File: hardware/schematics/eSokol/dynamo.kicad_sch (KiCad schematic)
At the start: 4 parts, among them U4 AMS1117-5.0

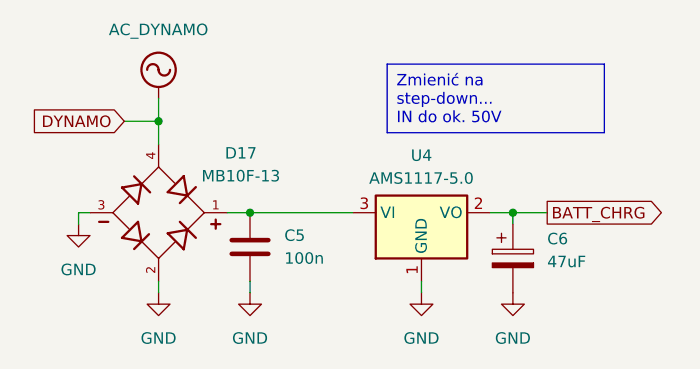
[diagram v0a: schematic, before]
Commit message: WIP: update some schematics to reflect the newest design changes
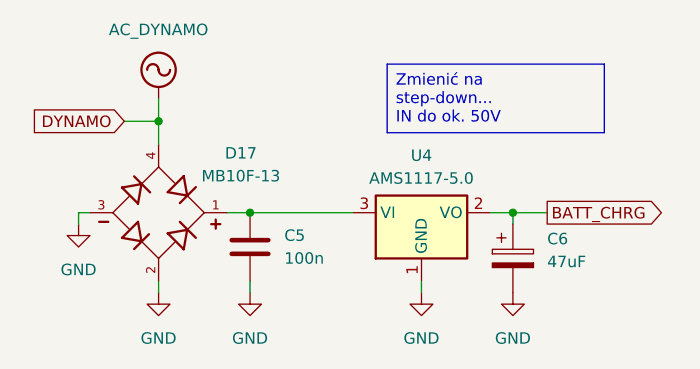
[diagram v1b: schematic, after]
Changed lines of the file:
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@@
 (kicad_sch
-	(version 20231120)
+	(version 20250114)
 	(generator "eeschema")
-	(generator_version "8.0")
+	(generator_version "9.0")
 	(paper "A4")
+	(text_box "Zmienić na step-down...\nIN do ok. 50V"
+		(exclude_from_sim no)
+		(at 115.57 69.85 0)
+		(size 24.13 7.62)
+		(margins 0.9525 0.9525 0.9525 0.9525)
+		(stroke
+			(width 0)
+			(type default)
+		)
+		(fill
+			(type none)
+		)
+		(effects
+			(font
+				(size 1.27 1.27)
+			)
+			(justify left top)
+		)
+	)
 	(junction
 		(at 129.54 86.36)
@@
 		)
 	)
-	(text_box "Zmienić na step-down...\nIN do ok. 50V"
-		(exclude_from_sim no)
-		(at 115.57 69.85 0)
-		(size 24.13 7.62)
-		(stroke
-			(width 0)
-			(type default)
-		)
-		(fill
-			(type none)
-		)
-		(effects
-			(font
-				(size 1.27 1.27)
-			)
-			(justify left top)
-		)
-	)
